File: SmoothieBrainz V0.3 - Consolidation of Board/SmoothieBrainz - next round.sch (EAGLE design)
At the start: 240 parts, among them IC1 LPC1769, IC5 LD117ADT33TR, Q1 BSL207SP, Q2 12MHz, Q3 25MHz, SW1 SW_TACT_4P_B, SW3 SW_TACT_4P_B, U2 HC_05, U3 USD-SOCKETUSD, X14 USBPTH, X2 GMSTBA2, X3 GMSTBA4, X4 1751248, X5 1751248, X6 1751248, X7 1751248, X8 1751248

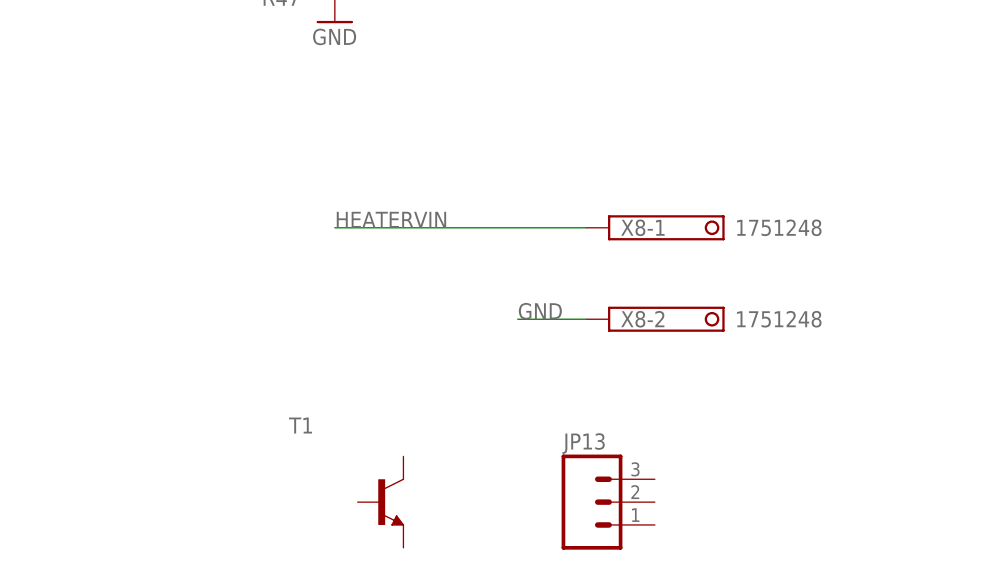
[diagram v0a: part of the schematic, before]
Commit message: Cleanup, first public preview.
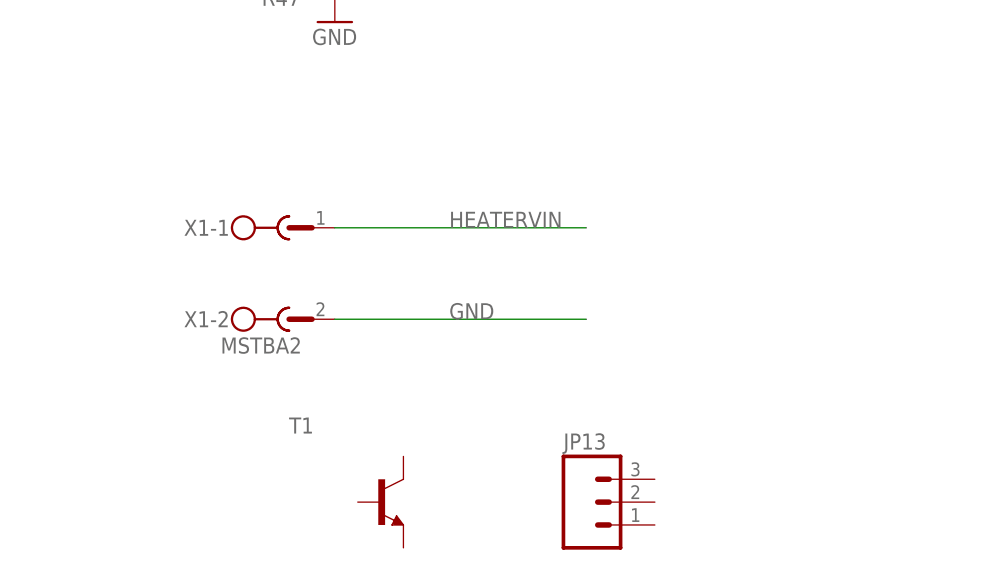
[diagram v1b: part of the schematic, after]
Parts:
- removed X8: 1751248, con-phoenix-350:1751248
- added X1: MSTBA2, con-phoenix-508:MSTBA2
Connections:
- net GND: now also X1-2.1; no longer X8-2.K
- net HEATERVIN: now also X1-1.1; no longer X8-1.K
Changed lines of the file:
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@@
 <part name="X6" library="con-phoenix-350" deviceset="1751248" device=""/>
 <part name="X7" library="con-phoenix-350" deviceset="1751248" device=""/>
-<part name="X8" library="con-phoenix-350" deviceset="1751248" device=""/>
 <part name="U$7" library="RepRapjr" deviceset="POLOLU_A4983CARRIER" device=""/>
 <part name="C38" library="resistor" deviceset="C-EU" device="C0603" value="104"/>
@@
 <part name="JP15" library="SparkFun-Connectors" deviceset="M03" device="LOCK"/>
 <part name="JP16" library="SparkFun-Connectors" deviceset="M03" device="LOCK"/>
+<part name="X1" library="con-phoenix-508" deviceset="MSTBA2" device=""/>
 </parts>
 <sheets>
@@
 <instance part="X7" gate="-1" x="553.72" y="233.68"/>
 <instance part="X7" gate="-2" x="553.72" y="226.06"/>
-<instance part="X8" gate="-1" x="551.18" y="187.96"/>
-<instance part="X8" gate="-2" x="551.18" y="177.8"/>
 <instance part="U$7" gate="G$1" x="347.98" y="124.46"/>
 <instance part="C38" gate="G$1" x="373.38" y="127" rot="R90"/>
@@
 <instance part="JP15" gate="G$1" x="548.64" y="127"/>
 <instance part="JP16" gate="G$1" x="548.64" y="111.76"/>
+<instance part="X1" gate="-1" x="515.62" y="187.96"/>
+<instance part="X1" gate="-2" x="515.62" y="177.8"/>
 </instances>
 <busses>
@@
 </segment>
 <segment>
-<pinref part="X8" gate="-2" pin="K"/>
-<wire x1="548.64" y1="177.8" x2="541.02" y2="177.8" width="0.1524" layer="91"/>
-<label x="541.02" y="177.8" size="1.778" layer="95"/>
+<wire x1="548.64" y1="177.8" x2="520.7" y2="177.8" width="0.1524" layer="91"/>
+<label x="533.4" y="177.8" size="1.778" layer="95"/>
+<pinref part="X1" gate="-2" pin="1"/>
 </segment>
 <segment>
@@
 <net name="HEATERVIN" class="0">
 <segment>
-<pinref part="X8" gate="-1" pin="K"/>
 <wire x1="548.64" y1="187.96" x2="520.7" y2="187.96" width="0.1524" layer="91"/>
-<label x="520.7" y="187.96" size="1.778" layer="95"/>
+<label x="533.4" y="187.96" size="1.778" layer="95"/>
+<pinref part="X1" gate="-1" pin="1"/>
 </segment>
 <segment>
